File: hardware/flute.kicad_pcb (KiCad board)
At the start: 2 copper layers, 230 x 20 mm, 34 parts, among them J1 Conn_01x04, J4 Conn_01x02, SW1 C, SW2 D, SW3 E, SW4 F, SW5 G, SW6 A, SW7 H, SW8 OCTAVE?, U1 W25Q128JVS, Y1 Crystal_GND24

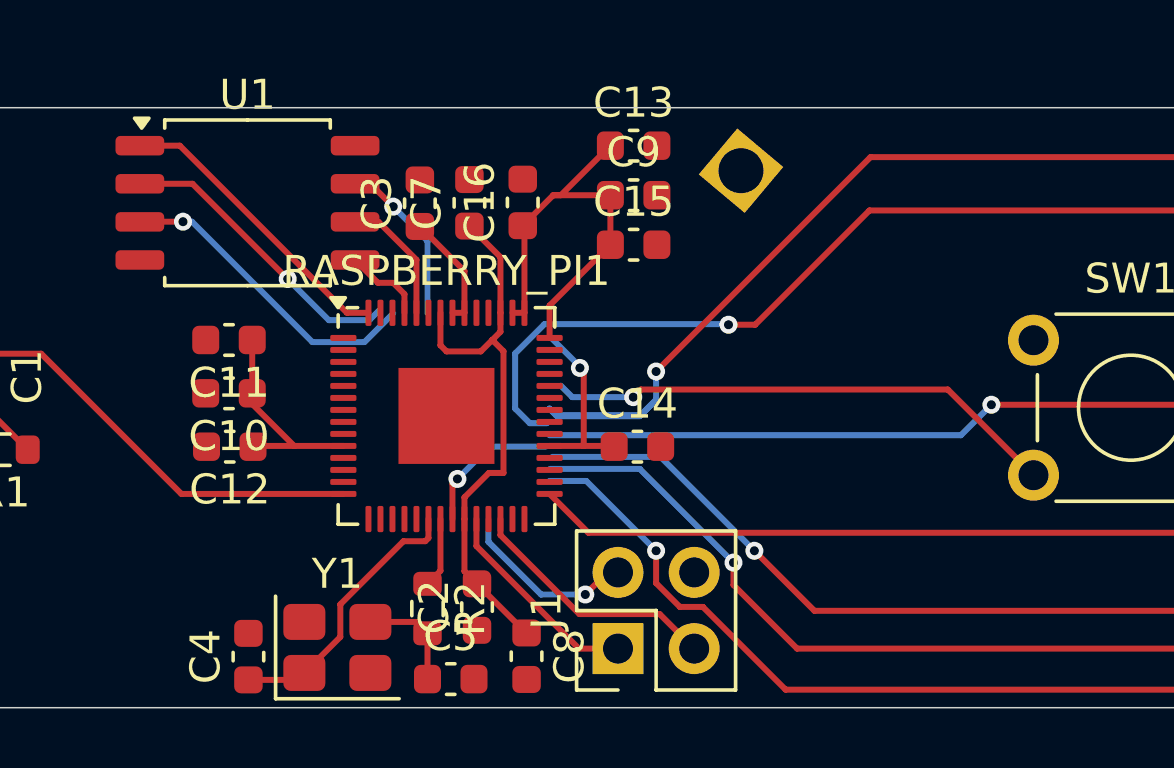
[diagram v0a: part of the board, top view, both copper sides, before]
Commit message: pcb connections corrected
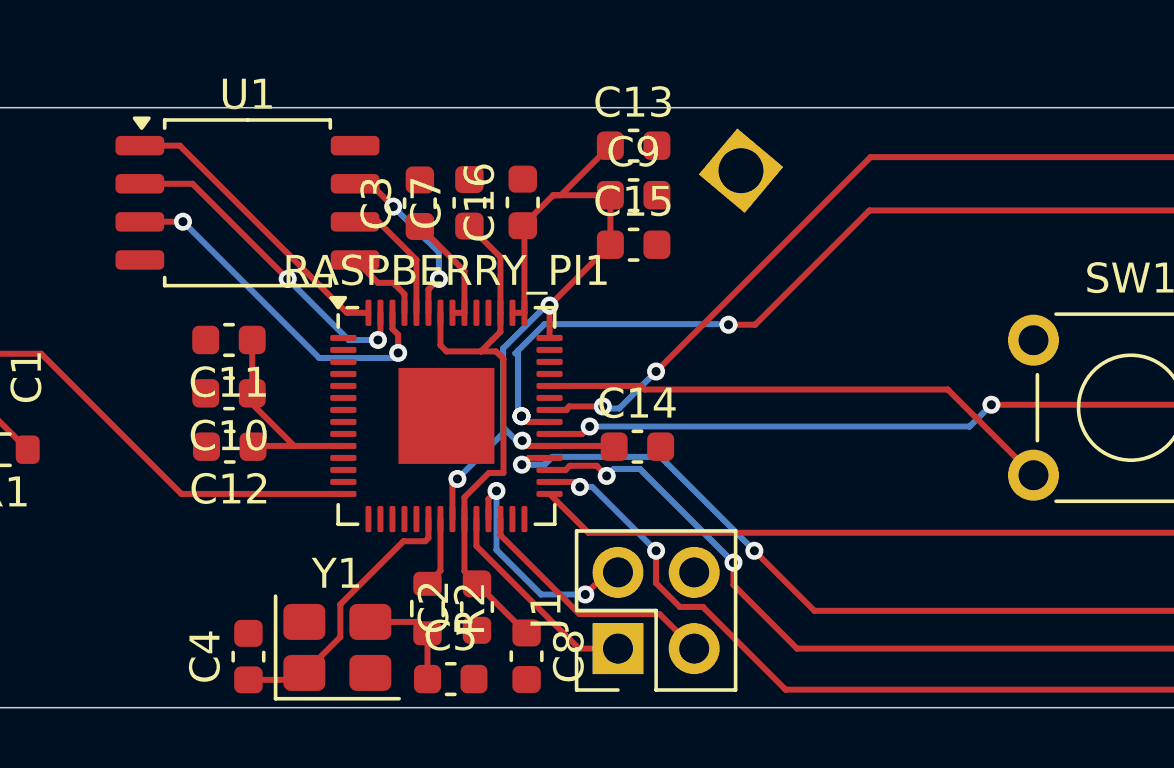
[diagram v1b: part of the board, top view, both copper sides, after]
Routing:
- net GPIO24: track 218.7 -> 214.2 mm, vias 1 -> 2
- net GPIO21: track 118.2 -> 120.3 mm, vias 1 -> 2
- net /RASPBERRY_PI_PICO/SWDIO: track 6.11 -> 7.98 mm, vias 1 -> 2
- net /RASPBERRY_PI_PICO/QSPI_SD2: track 10.5 -> 12.0 mm, vias 1 -> 2
- net +3V3: track 37.0 -> 38.4 mm, vias 2 -> 3
- net /RASPBERRY_PI_PICO/QSPI_SD1: track 9.99 -> 11.0 mm, vias 1 -> 2
- net /RASPBERRY_PI_PICO/QSPI_SD3: track 5.62 -> 5.99 mm, vias 1 -> 2
- net GPIO20: track 150.1 -> 150.4 mm, vias 1 -> 2
- net GPIO26: track 17.2 -> 17.4 mm, vias 1 -> 0
- net GPIO23: track 93.6 -> 93.8 mm, vias 1 -> 3
- net GPIO22: track 54.6 -> 54.5 mm, vias 1 -> 2
- net GPIO19: vias 1 -> 2
